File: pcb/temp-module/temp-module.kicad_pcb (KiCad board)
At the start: 2 copper layers, 37 x 27 mm, 18 parts, among them J1 Connector_male, J2 Screw_Terminal_01x03, U1 MCP6002-xP

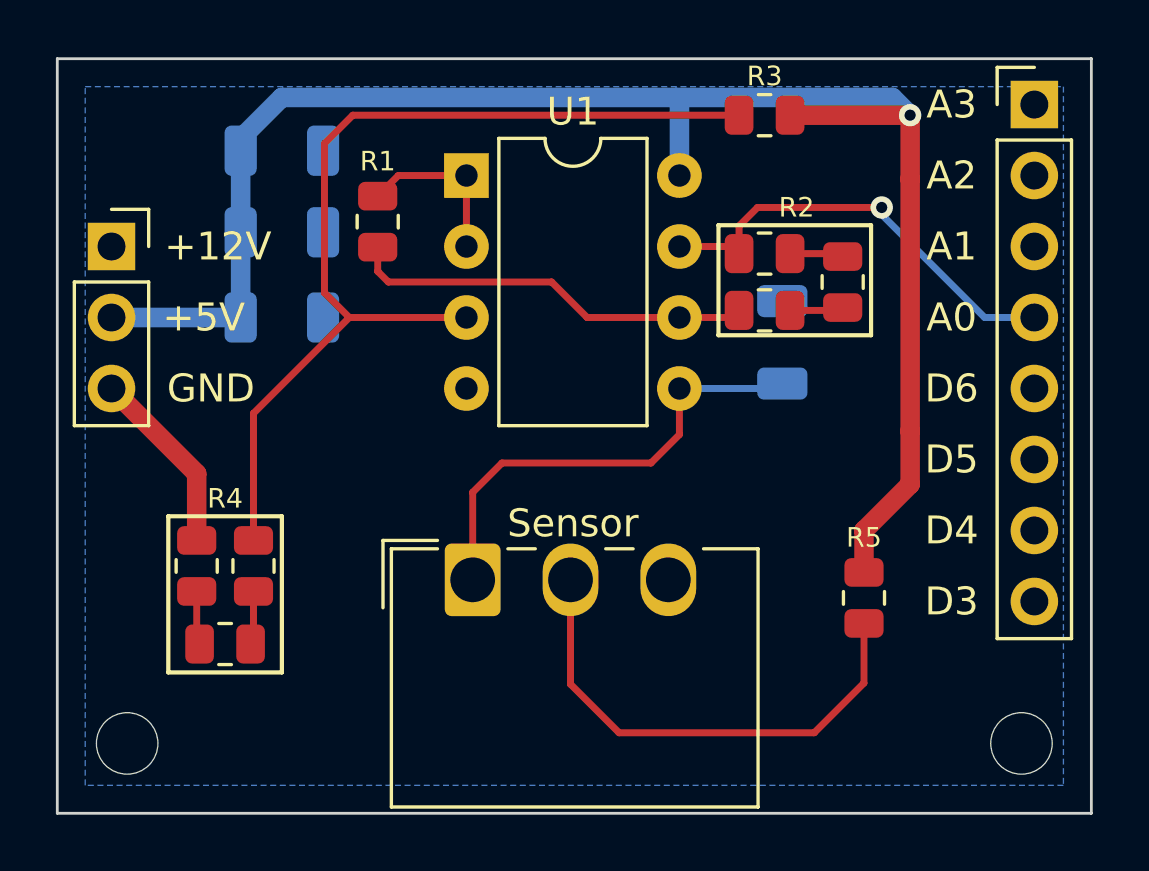
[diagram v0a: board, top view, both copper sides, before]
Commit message: pcb update
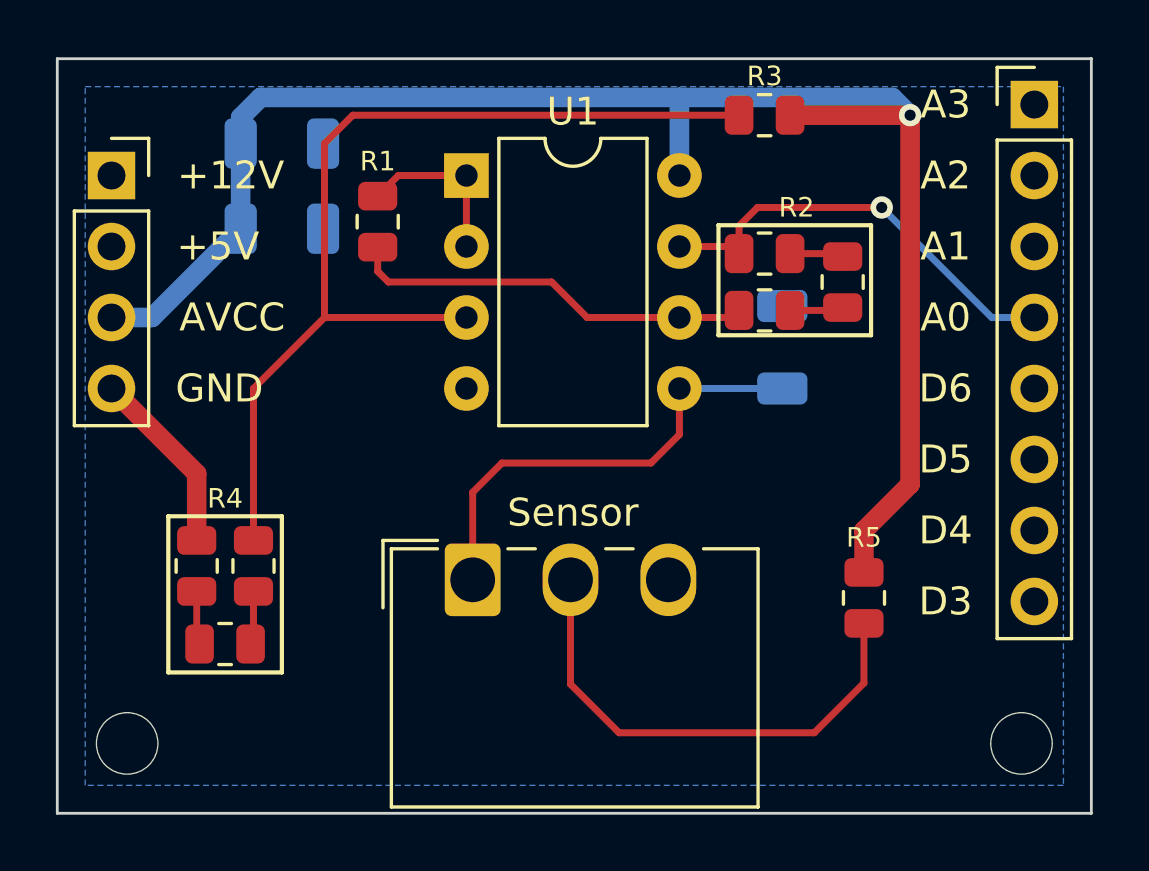
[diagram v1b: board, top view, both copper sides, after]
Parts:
- removed C3: 10uF/16V, Capacitor_SMD:C_1206_3216Metric
- C1: value 100nF -> 10uF/16V
- J1: value Connector_male -> Connector_male_4x8; footprint CAN_ATmega:Connector_male -> CAN_ATmega:Connector_male_4x8
- moved C1 3.17 mm to (148.3, 95.9)
- moved C2 3.17 mm to (148.3, 92.8), turned to 0 degrees
- moved J1 1.27 mm to (158.8, 99.1)
- moved C4 0.18 mm to (166.2, 100.1)
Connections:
- C1 pad 1: +5V -> AVCC
- C2 pad 1: GND -> AVCC
- C2 pad 2: +5V -> GND
- J1 pad 2: +5V -> unconnected-(J1-Pad2)
- J1 pad 3: GND -> AVCC
- J1 pad 4: unconnected-(J1-Pad4) -> GND
- J1 pad 8: SREG -> unconnected-(J1-Pad8)
- J1 pad 9: unconnected-(J1-Pad9) -> SREG
- R3 pad 1: +5V -> AVCC
- R5 pad 2: +5V -> AVCC
- U1 pad 8: +5V -> AVCC
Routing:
- net +5V: track 60.0 -> 0.00 mm, vias 1 -> 0
- net AVCC: track 0.00 -> 58.6 mm, vias 0 -> 1
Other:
- board text removed: "GND"
